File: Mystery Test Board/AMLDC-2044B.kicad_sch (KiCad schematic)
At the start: 331 parts, among them J1 Port A, J2 Port B, Q1 PNP MPS6533, Y1 Crystal

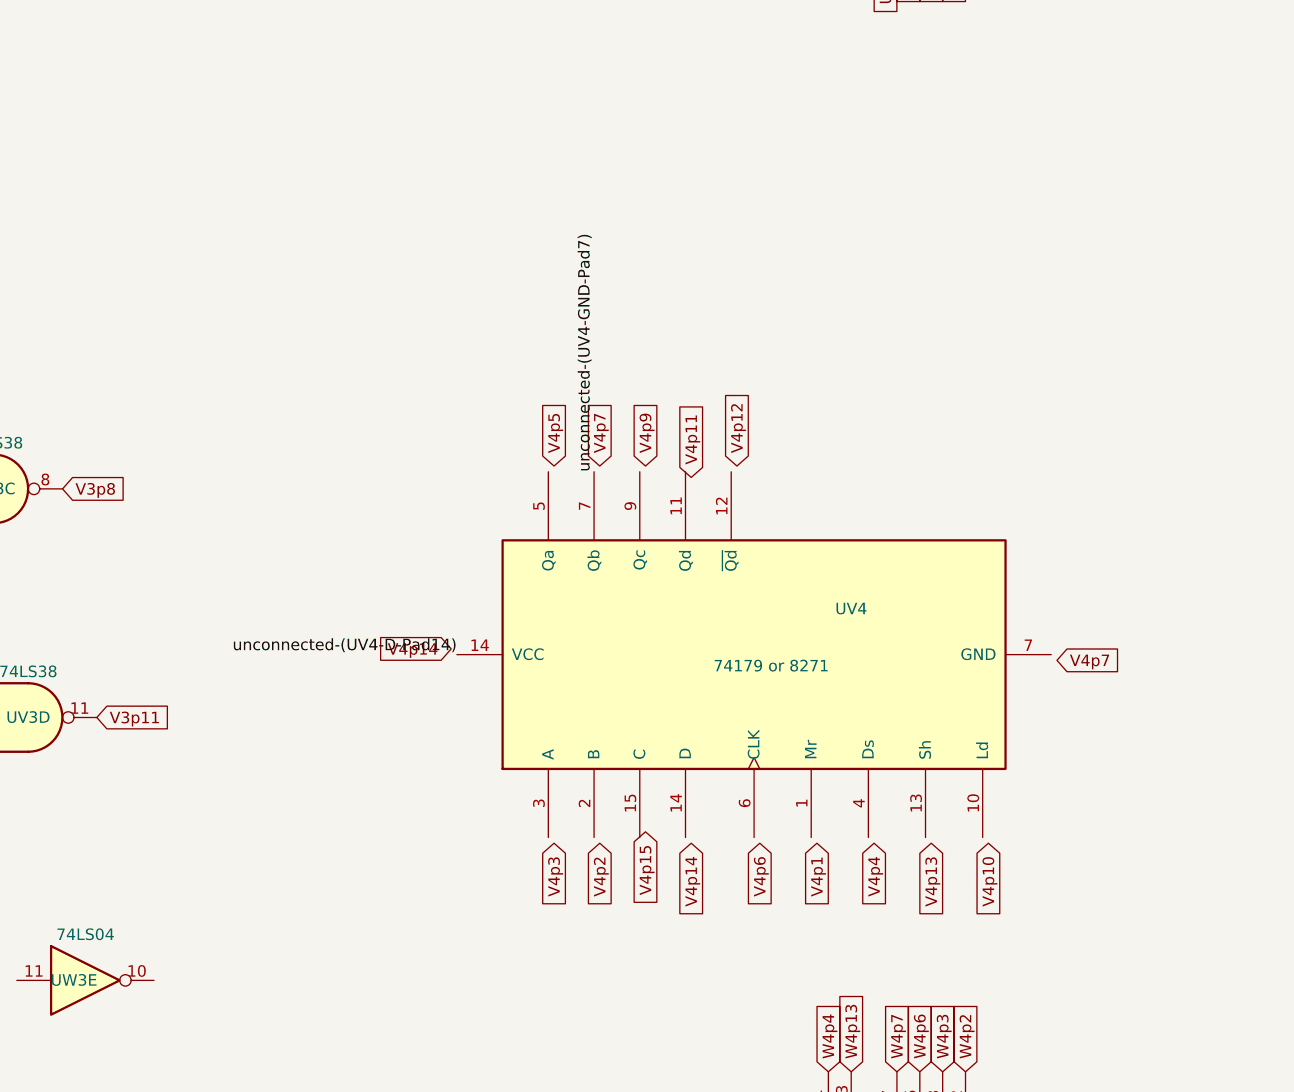
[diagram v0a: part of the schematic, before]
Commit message: Trace Part 3
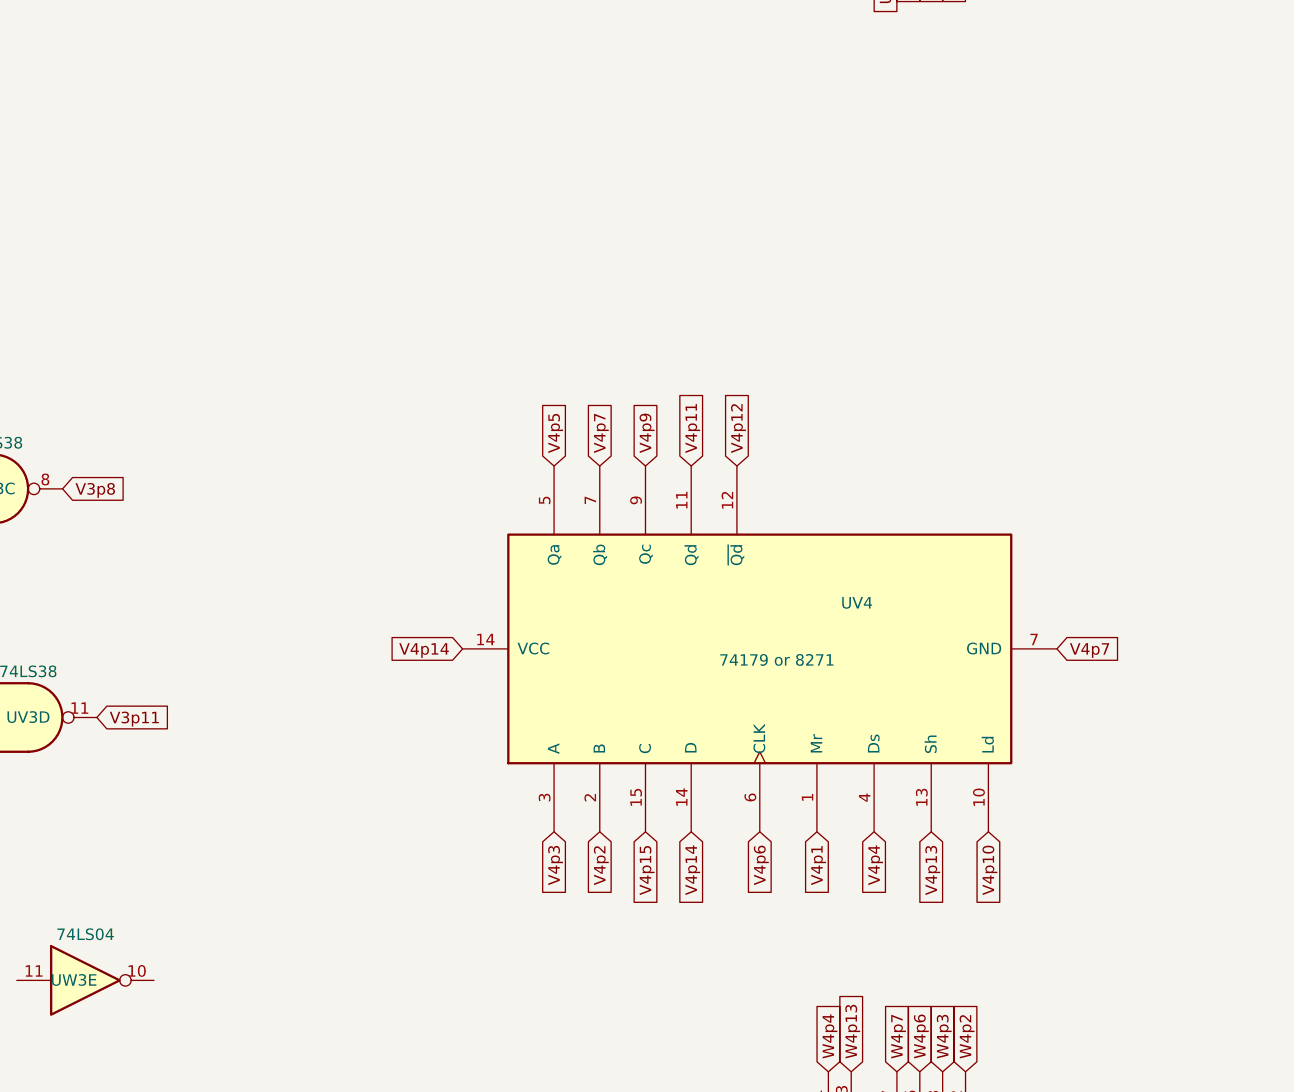
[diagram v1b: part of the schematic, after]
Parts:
- UU4, UV4: footprint Package_DIP:DIP-16_W7.62mm -> Package_DIP:DIP-14_W7.62mm
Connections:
- net unconnected-(UV4-D-Pad14) is gone; now on net V4p14: UV4.14 (D)
- net unconnected-(UV4-GND-Pad7) is gone; now on net V4p7: UV4.7 (Qb)
- net V4p1: now also UV4.1 (Mr)
- net V4p10: now also UV4.10 (Ld)
- net V4p11: now also UV4.11 (Qd)
- net V4p12: now also UV4.12 (~{Qd})
- net V4p13: now also UV4.13 (Sh)
- net V4p15: now also UV4.15 (C)
- net V4p2: now also UV4.2 (B)
- net V4p3: now also UV4.3 (A)
- net V4p4: now also UV4.4 (Ds)
- net V4p5: now also UV4.5 (Qa)
- net V4p6: now also UV4.6 (CLK)
- net V4p9: now also UV4.9 (Qc)
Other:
- moved on the sheet: UV4
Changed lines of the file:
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@@
     (effects (font (size 1.27 1.27)) (justify right bottom))
   )
-  (label "GND" (at 553.085 1157.605 180)
+  (label "GND" (at 553.085 1157.605 180) (fields_autoplaced)
     (effects (font (size 1.27 1.27)) (justify right bottom))
   )
@@
     (effects (font (size 1.27 1.27)) (justify right bottom))
   )
-  (label "GND" (at 218.44 162.56 180)
+  (label "GND" (at 218.44 162.56 180) (fields_autoplaced)
     (effects (font (size 1.27 1.27)) (justify right bottom))
   )
@@
     (effects (font (size 1.27 1.27)) (justify right bottom))
   )
-  (label "GND" (at 201.93 236.22 0)
+  (label "GND" (at 201.93 236.22 0) (fields_autoplaced)
     (effects (font (size 1.27 1.27)) (justify left bottom))
   )
@@
     (effects (font (size 1.27 1.27)) (justify right bottom))
   )
-  (label "unconnected-(UV4-D-Pad14)" (at 657.225 1207.135 180) (fields_autoplaced)
-    (effects (font (size 1.27 1.27)) (justify right bottom))
-  )
   (label "Net-(UG4A-Q)" (at 757.555 372.11 0) (fields_autoplaced)
     (effects (font (size 1.27 1.27)) (justify left bottom))
@@
     (effects (font (size 1.27 1.27)) (justify right bottom))
   )
-  (label "unconnected-(UV4-GND-Pad7)" (at 672.465 1186.815 90)
-    (effects (font (size 1.27 1.27)) (justify left bottom))
-  )
   (label "+5V" (at -127 207.01 90) (fields_autoplaced)
     (effects (font (size 1.27 1.27)) (justify left bottom))
@@
     (effects (font (size 1.27 1.27)) (justify right bottom))
   )
-  (label "+5V" (at 565.785 1157.605 0)
+  (label "+5V" (at 565.785 1157.605 0) (fields_autoplaced)
     (effects (font (size 1.27 1.27)) (justify left bottom))
   )
@@
     )
   )
-  (global_label "V4p4" (shape input) (at 703.58 1228.09 270) (fields_autoplaced)
+  (global_label "V4p4" (shape input) (at 703.58 1226.82 270) (fields_autoplaced)
     (effects (font (size 1.27 1.27)) (justify right))
-    (property "Intersheetrefs" "${INTERSHEET_REFS}" (at 703.58 1235.7318 90)
+    (property "Intersheetrefs" "${INTERSHEET_REFS}" (at 703.58 1234.4618 90)
       (effects (font (size 1.27 1.27)) (justify right) hide)
     )
@@
     )
   )
-  (global_label "V4p14" (shape input) (at 656.59 1206.5 180) (fields_autoplaced)
+  (global_label "V4p14" (shape input) (at 657.86 1206.5 180) (fields_autoplaced)
     (effects (font (size 1.27 1.27)) (justify right))
-    (property "Intersheetrefs" "${INTERSHEET_REFS}" (at 647.7387 1206.5 0)
+    (property "Intersheetrefs" "${INTERSHEET_REFS}" (at 649.0087 1206.5 0)
       (effects (font (size 1.27 1.27)) (justify right) hide)
     )
@@
     )
   )
-  (global_label "V4p13" (shape input) (at 709.93 1228.09 270) (fields_autoplaced)
+  (global_label "V4p13" (shape input) (at 709.93 1226.82 270) (fields_autoplaced)
     (effects (font (size 1.27 1.27)) (justify right))
-    (property "Intersheetrefs" "${INTERSHEET_REFS}" (at 709.93 1236.9413 90)
+    (property "Intersheetrefs" "${INTERSHEET_REFS}" (at 709.93 1235.6713 90)
       (effects (font (size 1.27 1.27)) (justify right) hide)
     )
@@
     )
   )
-  (global_label "V4p3" (shape input) (at 668.02 1228.09 270) (fields_autoplaced)
+  (global_label "V4p3" (shape input) (at 668.02 1226.82 270) (fields_autoplaced)
     (effects (font (size 1.27 1.27)) (justify right))
-    (property "Intersheetrefs" "${INTERSHEET_REFS}" (at 668.02 1235.7318 90)
+    (property "Intersheetrefs" "${INTERSHEET_REFS}" (at 668.02 1234.4618 90)
       (effects (font (size 1.27 1.27)) (justify right) hide)
     )
@@
     )
   )
-  (global_label "V4p7" (shape input) (at 723.9 1207.77 0) (fields_autoplaced)
+  (global_label "V4p7" (shape input) (at 723.9 1206.5 0) (fields_autoplaced)
     (effects (font (size 1.27 1.27)) (justify left))
-    (property "Intersheetrefs" "${INTERSHEET_REFS}" (at 731.5418 1207.77 0)
+    (property "Intersheetrefs" "${INTERSHEET_REFS}" (at 731.5418 1206.5 0)
       (effects (font (size 1.27 1.27)) (justify left) hide)
     )
@@
     )
   )
-  (global_label "V4p1" (shape input) (at 697.23 1228.09 270) (fields_autoplaced)
+  (global_label "V4p1" (shape input) (at 697.23 1226.82 270) (fields_autoplaced)
     (effects (font (size 1.27 1.27)) (justify right))
-    (property "Intersheetrefs" "${INTERSHEET_REFS}" (at 697.23 1235.7318 90)
+    (property "Intersheetrefs" "${INTERSHEET_REFS}" (at 697.23 1234.4618 90)
       (effects (font (size 1.27 1.27)) (justify right) hide)
     )
@@
     )
   )
-  (global_label "V4p14" (shape input) (at 683.26 1228.09 270) (fields_autoplaced)
+  (global_label "V4p14" (shape input) (at 683.26 1226.82 270) (fields_autoplaced)
     (effects (font (size 1.27 1.27)) (justify right))
-    (property "Intersheetrefs" "${INTERSHEET_REFS}" (at 683.26 1236.9413 90)
+    (property "Intersheetrefs" "${INTERSHEET_REFS}" (at 683.26 1235.6713 90)
       (effects (font (size 1.27 1.27)) (justify right) hide)
     )
@@
     )
   )
-  (global_label "V4p10" (shape input) (at 716.28 1228.09 270) (fields_autoplaced)
+  (global_label "V4p10" (shape input) (at 716.28 1226.82 270) (fields_autoplaced)
     (effects (font (size 1.27 1.27)) (justify right))
-    (property "Intersheetrefs" "${INTERSHEET_REFS}" (at 716.28 1236.9413 90)
+    (property "Intersheetrefs" "${INTERSHEET_REFS}" (at 716.28 1235.6713 90)
       (effects (font (size 1.27 1.27)) (justify right) hide)
     )
@@
     )
   )
-  (global_label "V4p2" (shape input) (at 673.1 1228.09 270) (fields_autoplaced)
+  (global_label "V4p2" (shape input) (at 673.1 1226.82 270) (fields_autoplaced)
     (effects (font (size 1.27 1.27)) (justify right))
-    (property "Intersheetrefs" "${INTERSHEET_REFS}" (at 673.1 1235.7318 90)
+    (property "Intersheetrefs" "${INTERSHEET_REFS}" (at 673.1 1234.4618 90)
       (effects (font (size 1.27 1.27)) (justify right) hide)
     )
@@
     )
   )
-  (global_label "V4p11" (shape input) (at 683.26 1187.45 90) (fields_autoplaced)
+  (global_label "V4p11" (shape input) (at 683.26 1186.18 90) (fields_autoplaced)
     (effects (font (size 1.27 1.27)) (justify left))
-    (property "Intersheetrefs" "${INTERSHEET_REFS}" (at 683.26 1178.5987 90)
+    (property "Intersheetrefs" "${INTERSHEET_REFS}" (at 683.26 1177.3287 90)
       (effects (font (size 1.27 1.27)) (justify left) hide)
     )
@@
     )
   )
-  (global_label "V4p6" (shape input) (at 690.88 1228.09 270) (fields_autoplaced)
+  (global_label "V4p6" (shape input) (at 690.88 1226.82 270) (fields_autoplaced)
     (effects (font (size 1.27 1.27)) (justify right))
-    (property "Intersheetrefs" "${INTERSHEET_REFS}" (at 690.88 1235.7318 90)
+    (property "Intersheetrefs" "${INTERSHEET_REFS}" (at 690.88 1234.4618 90)
       (effects (font (size 1.27 1.27)) (justify right) hide)
     )
@@
       (effects (font (size 1.27 1.27)))
     )
-    (property "Footprint" "Package_DIP:DIP-16_W7.62mm" (at 699.77 1115.06 0)
+    (property "Footprint" "Package_DIP:DIP-14_W7.62mm" (at 699.77 1115.06 0)
       (effects (font (size 1.27 1.27)) hide)
     )
@@
     )
   )
-  (symbol (lib_id "ForgottenMachines:74179") (at 690.245 1207.135 90) (unit 1)
+  (symbol (lib_id "ForgottenMachines:74179") (at 690.88 1206.5 90) (unit 1)
     (in_bom yes) (on_board yes) (dnp no)
-    (property "Reference" "UV4" (at 701.04 1202.055 90)
+    (property "Reference" "UV4" (at 701.675 1201.42 90)
       (effects (font (size 1.27 1.27)))
     )
-    (property "Value" "74179\n or\n8271" (at 692.15 1208.405 90)
+    (property "Value" "74179\n or\n8271" (at 692.785 1207.77 90)
       (effects (font (size 1.27 1.27)))
     )
-    (property "Footprint" "Package_DIP:DIP-16_W7.62mm" (at 706.755 1170.305 0)
+    (property "Footprint" "Package_DIP:DIP-14_W7.62mm" (at 707.39 1169.67 0)
       (effects (font (size 1.27 1.27)) hide)
     )
-    (property "Datasheet" "" (at 685.165 1207.135 0)
+    (property "Datasheet" "" (at 685.8 1206.5 0)
       (effects (font (size 1.27 1.27)) hide)
     )
